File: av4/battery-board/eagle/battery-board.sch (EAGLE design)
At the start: 57 parts, among them J100 ROCKETNET-BATTERY-14, J101 87758-0216, J102 87758-0216, Q100 Si2343DS-T1, Q101 SI4435DDY, Q102 SI4435DDY, Q103 SI1023X, Q104 SI1023X, U100 BQ3060PW

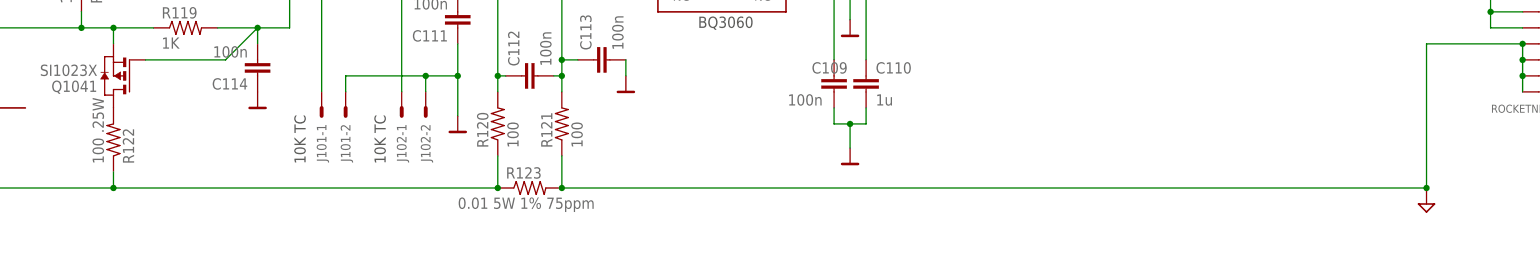
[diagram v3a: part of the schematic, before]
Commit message: Final cleanup on battery board. Made stitching more focused on power rather than RF, redid shunt library part to be a real kelvin connection (see Analog Devices cute write up on Kelvin sense shunt resistors), changes all polygons to be consistenly 0.2 mm wid and 0.2 mm isolate.
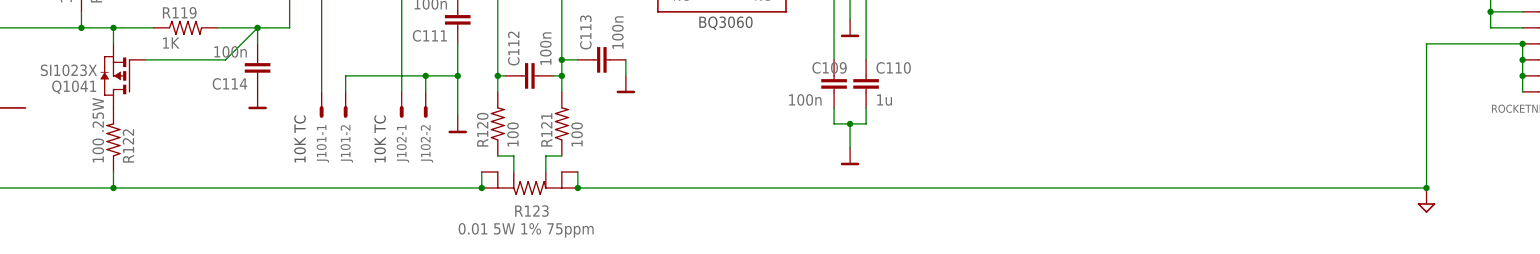
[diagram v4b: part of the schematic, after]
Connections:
- new net N$16: R121.1, R123.K2
- new net N$3: R120.1, R123.K1
- net BAR_GND: now also R123.1@1, R123.1@2; no longer R120.1, R123.1
- net TRIANGLE_GND: now also R123.2@1, R123.2@2; no longer R121.1, R123.2
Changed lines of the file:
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@@
 <?xml version="1.0" encoding="utf-8"?>
 <!DOCTYPE eagle SYSTEM "eagle.dtd">
-<eagle version="6.4">
+<eagle version="6.5.0">
 <drawing>
 <settings>
@@
 <setting verticaltext="up"/>
 </settings>
-<grid distance="0.1" unitdist="inch" unit="inch" style="lines" multiple="1" display="no" altdistance="0.01" altunitdist="inch" altunit="inch"/>
+<grid distance="0.05" unitdist="inch" unit="inch" style="lines" multiple="2" display="no" altdistance="0.01" altunitdist="inch" altunit="inch"/>
 <layers>
 <layer number="1" name="Top" color="4" fill="1" visible="no" active="no"/>
@@
 <part name="J101" library="con-molex" deviceset="87758-0216" device=""/>
 <part name="J102" library="con-molex" deviceset="87758-0216" device=""/>
-<part name="R123" library="shunt" deviceset="R-US-2818" device="" value="0.01 5W 1% 75ppm"/>
 <part name="R120" library="rcl_custom" deviceset="R-US_" device="0603-B-NOSILK" value="100"/>
 <part name="R121" library="rcl_custom" deviceset="R-US_" device="0603-B-NOSILK" value="100"/>
@@
 <part name="C118" library="rcl_custom" deviceset="C-EU" device="0603-B-NOSILK" value="100n/50V"/>
 <part name="Q100" library="Tova" deviceset="NTR4101P" device="" value="Si2343DS-T1"/>
+<part name="R123" library="shunt" deviceset="R-US-2818" device="" value="0.01 5W 1% 75ppm"/>
 </parts>
 <sheets>
@@
 <instance part="J102" gate="-2" x="151.13" y="101.6" smashed="yes" rot="R270">
 <attribute name="NAME" x="150.368" y="99.06" size="1.524" layer="95" rot="R270"/>
-</instance>
-<instance part="R123" gate="G$1" x="167.64" y="88.9" smashed="yes">
-<attribute name="NAME" x="163.83" y="90.3986" size="1.778" layer="95"/>
-<attribute name="VALUE" x="156.21" y="85.598" size="1.778" layer="96"/>
 </instance>
 <instance part="R120" gate="R" x="162.56" y="99.06" rot="R90"/>
@@
 <attribute name="NAME" x="218.44" y="237.49" size="1.778" layer="95" rot="MR180"/>
 </instance>
+<instance part="R123" gate="G$1" x="167.64" y="88.9" smashed="yes" rot="MR180">
+<attribute name="NAME" x="165.1" y="86.1314" size="1.778" layer="95" rot="MR180"/>
+<attribute name="VALUE" x="156.21" y="83.312" size="1.778" layer="96" rot="MR180"/>
+</instance>
 </instances>
 <busses>
@@
 <wire x1="101.6" y1="88.9" x2="78.74" y2="88.9" width="1.27" layer="91"/>
 <wire x1="101.6" y1="91.44" x2="101.6" y2="88.9" width="0.1524" layer="91"/>
-<wire x1="162.56" y1="88.9" x2="101.6" y2="88.9" width="1.27" layer="91"/>
-<wire x1="162.56" y1="93.98" x2="162.56" y2="88.9" width="0.1524" layer="91"/>
+<wire x1="160.02" y1="88.9" x2="101.6" y2="88.9" width="1.27" layer="91"/>
 <wire x1="78.74" y1="88.9" x2="78.74" y2="96.52" width="1.27" layer="91"/>
 <junction x="101.6" y="88.9"/>
-<junction x="162.56" y="88.9"/>
 <junction x="78.74" y="88.9"/>
 <pinref part="BAR_GND7" gate="1" pin="BAR_GND"/>
 <pinref part="R122" gate="R" pin="1"/>
-<pinref part="R123" gate="G$1" pin="1"/>
-<pinref part="R120" gate="R" pin="1"/>
 <pinref part="B100A" gate="G$1" pin="B-@1"/>
 <wire x1="77.47" y1="96.52" x2="78.74" y2="96.52" width="1.27" layer="91"/>
@@
 <wire x1="78.74" y1="96.52" x2="80.01" y2="96.52" width="1.27" layer="91"/>
 <junction x="78.74" y="96.52"/>
+<pinref part="R123" gate="G$1" pin="1@1"/>
+<junction x="160.02" y="88.9"/>
+<pinref part="R123" gate="G$1" pin="1@2"/>
+<wire x1="160.02" y1="88.9" x2="160.02" y2="91.44" width="1.27" layer="91"/>
 </segment>
 <segment>
@@
 <net name="TRIANGLE_GND" class="0">
 <segment>
-<wire x1="172.72" y1="93.98" x2="172.72" y2="88.9" width="0.1524" layer="91"/>
-<wire x1="172.72" y1="88.9" x2="309.88" y2="88.9" width="1.27" layer="91"/>
+<wire x1="175.26" y1="88.9" x2="309.88" y2="88.9" width="1.27" layer="91"/>
 <wire x1="309.88" y1="111.76" x2="309.88" y2="88.9" width="1.27" layer="91"/>
-<junction x="172.72" y="88.9"/>
 <junction x="309.88" y="88.9"/>
-<pinref part="R121" gate="R" pin="1"/>
-<pinref part="R123" gate="G$1" pin="2"/>
 <pinref part="TRIANGLE_GND3" gate="1" pin="TRIANGLE_GND"/>
 <pinref part="J100" gate="G$1" pin="B-@1"/>
@@
 <wire x1="325.12" y1="106.68" x2="325.12" y2="104.14" width="0.1524" layer="91"/>
 <junction x="325.12" y="106.68"/>
+<pinref part="R123" gate="G$1" pin="2@1"/>
+<junction x="175.26" y="88.9"/>
+<pinref part="R123" gate="G$1" pin="2@2"/>
+<wire x1="175.26" y1="91.44" x2="175.26" y2="88.9" width="1.27" layer="91"/>
 </segment>
 <segment>
@@
 </segment>
 </net>
+<net name="N$3" class="0">
+<segment>
+<pinref part="R120" gate="R" pin="1"/>
+<pinref part="R123" gate="G$1" pin="K1"/>
+<wire x1="162.56" y1="93.98" x2="165.1" y2="93.98" width="0.1524" layer="91"/>
+<wire x1="165.1" y1="93.98" x2="165.1" y2="91.44" width="0.1524" layer="91"/>
+</segment>
+</net>
+<net name="N$16" class="0">
+<segment>
+<pinref part="R121" gate="R" pin="1"/>
+<pinref part="R123" gate="G$1" pin="K2"/>
+<wire x1="172.72" y1="93.98" x2="170.18" y2="93.98" width="0.1524" layer="91"/>
+<wire x1="170.18" y1="93.98" x2="170.18" y2="91.44" width="0.1524" layer="91"/>
+</segment>
+</net>
